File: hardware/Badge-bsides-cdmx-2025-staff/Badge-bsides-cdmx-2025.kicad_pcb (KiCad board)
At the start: 2 copper layers, 50.1 x 110 mm, 44 parts, among them J1 SWDIO, J3 ADDON, J4 Conn_01x04_Pin, J5 I2C, J6 Conn_01x04_Pin, P6 USB_C_Plug_USB2.0, Q3 DMG3415U-7, SW10 SW_Push, SW11 ON, SW2 RESET, SW7 SW_Push, SW8 SW_Push, SW9 SW_Push, U1 PY32F030F28U6TR, U6 AP2112K-3.3

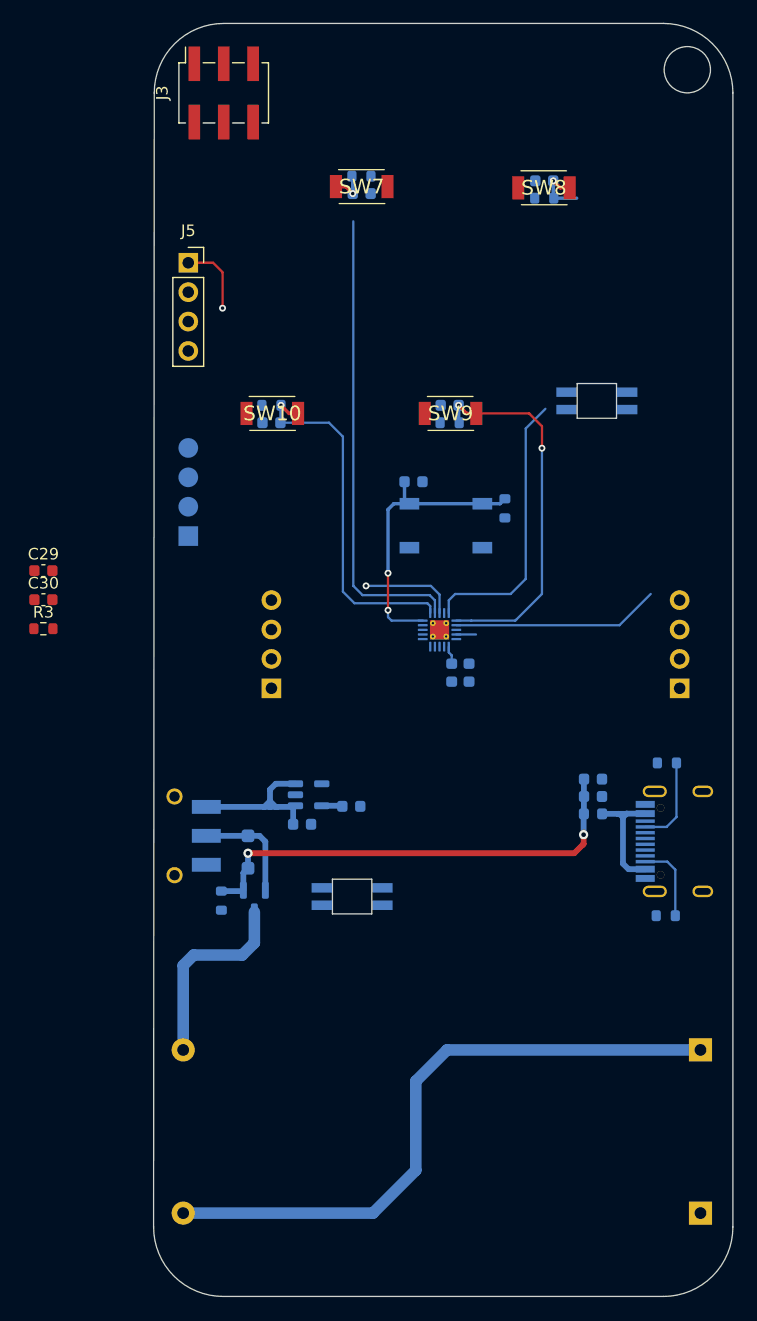
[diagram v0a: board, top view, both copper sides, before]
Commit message: feat(HW):Staff_Updated
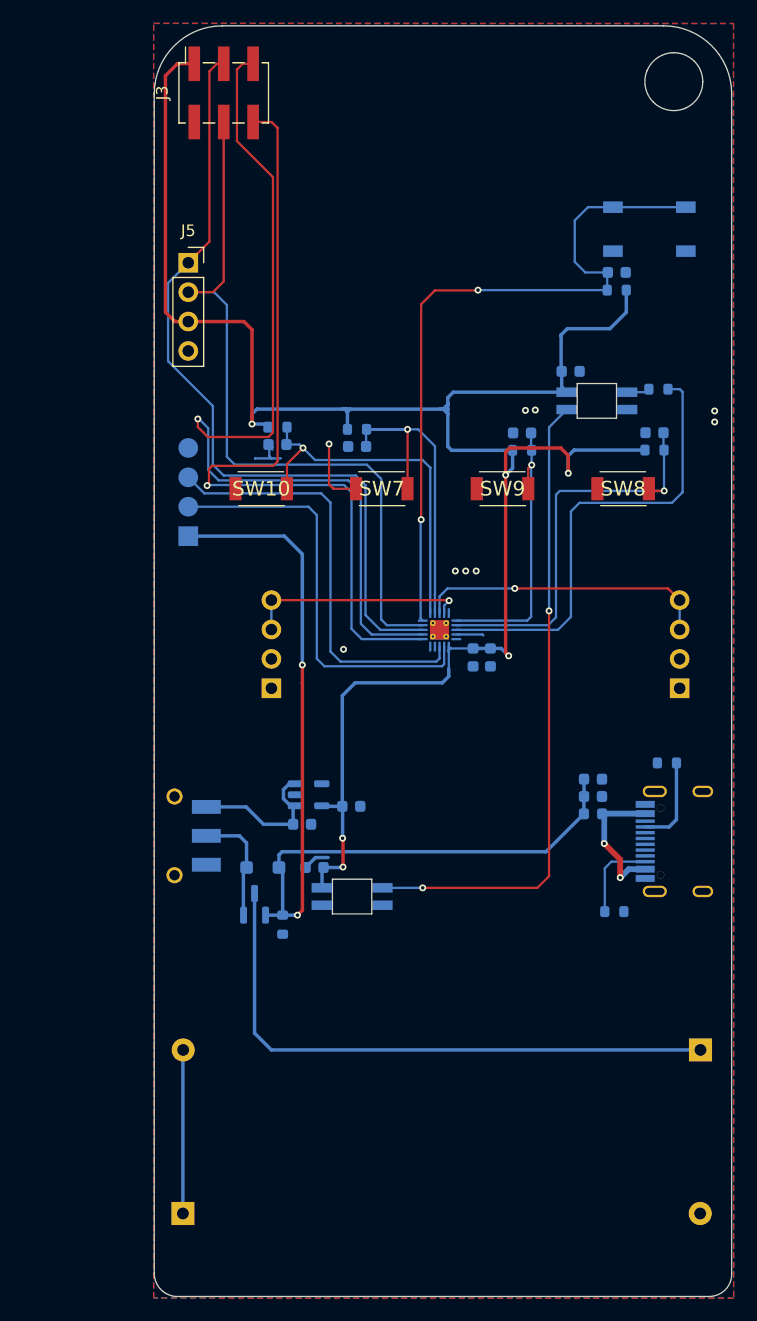
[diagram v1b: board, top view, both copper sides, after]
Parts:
- added kibuzzard-684362A9: G***, kibuzzard-684362A9, B.Cu at (110.5, 105.1)
- added kibuzzard-684362BF: G***, kibuzzard-684362BF, B.Cu at (108.6, 116.2)
- added kibuzzard-684362CB: G***, kibuzzard-684362CB, B.Cu at (114.7, 100.8)
- added kibuzzard-684362D8: G***, kibuzzard-684362D8, B.Cu at (151.2, 100.8)
- added kibuzzard-684362E4: G***, kibuzzard-684362E4, B.Cu at (148.1, 61.6)
- C29, C30, R3: moved to B.Cu
- moved R3 57.0 mm to (148.5, 71.6), turned to 180 degrees
- moved C29 48.7 mm to (140.9, 70.1)
- moved BT4 44.7 mm to (107.4, 142.9), turned to 0 degrees
- moved C30 32.9 mm to (118.8, 113.0), turned to 180 degrees
- moved SW2 31.1 mm to (147.7, 57.8)
- moved SW8 26.9 mm to (145.4, 80.2)
- moved SW7 26.2 mm to (124.6, 80.2), turned to 0 degrees
- moved C6 25.2 mm to (144.9, 61.5)
- moved C67 23.8 mm to (148.2, 75.4)
- moved R5 23.8 mm to (148.2, 76.9)
- moved R7 21.9 mm to (122.4, 75.1), turned to 180 degrees
- moved C69 21.9 mm to (122.5, 76.6), turned to 180 degrees
- moved R4 21.2 mm to (144.9, 63.1), turned to 0 degrees
- moved SW9 7.91 mm to (135.0, 80.2)
- moved C68 6.70 mm to (136.7, 75.4)
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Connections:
- BT4 pad 1: GND -> Net-(BT3--)
- BT4 pad 2: Net-(BT3--) -> GND
- J4 pad 3: /RX -> /TX
- J4 pad 4: /RX -> /TX
- J6 pad 3: /TX -> /RX
- J6 pad 4: /TX -> /RX
- U1 pad 10: /LED1 -> unconnected-(U1-PB6-Pad10)
- U1 pad 12: unconnected-(U1-PF4/BOOT0-Pad12) -> /GPIO2
- U1 pad 20: /LED2 -> unconnected-(U1-PA4-Pad20)
- U1 pad 5: /GPIO2 -> unconnected-(U1-PA12-Pad5)
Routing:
- net +3.3V: track 3.44 -> 171.4 mm, vias 0 -> 6
- net /GPIO2: track 0.00 -> 77.8 mm, vias 0 -> 1
- net /GPIO1: track 0.00 -> 69.9 mm, vias 0 -> 1
- net /SCL: track 0.03 -> 64.2 mm
- net /SDA: track 6.40 -> 69.2 mm, vias 1 -> 0
- net Net-(D19-DOUT): track 0.00 -> 55.8 mm, vias 0 -> 2
- net Net-(BT3--): track 55.1 -> 14.1 mm
- net VBUS: track 40.2 -> 80.8 mm
- net /NEO: track 0.00 -> 39.8 mm
- net /NTST: track 25.0 -> 62.5 mm
- net /SWCLK: track 0.00 -> 37.0 mm
- net /SWDIO: track 0.00 -> 36.7 mm
- net +BATT: track 16.9 -> 51.2 mm
- net /LED2: track 23.9 -> 0.00 mm
- net /RX: track 0.00 -> 19.2 mm, vias 0 -> 1
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- added copper zone on B.Cu, net GND
- added copper zone on F.Cu, net GND
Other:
- board size 50.1 x 110 mm -> 49.9 x 109.8 mm
